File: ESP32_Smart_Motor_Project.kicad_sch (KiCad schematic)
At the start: 14 parts

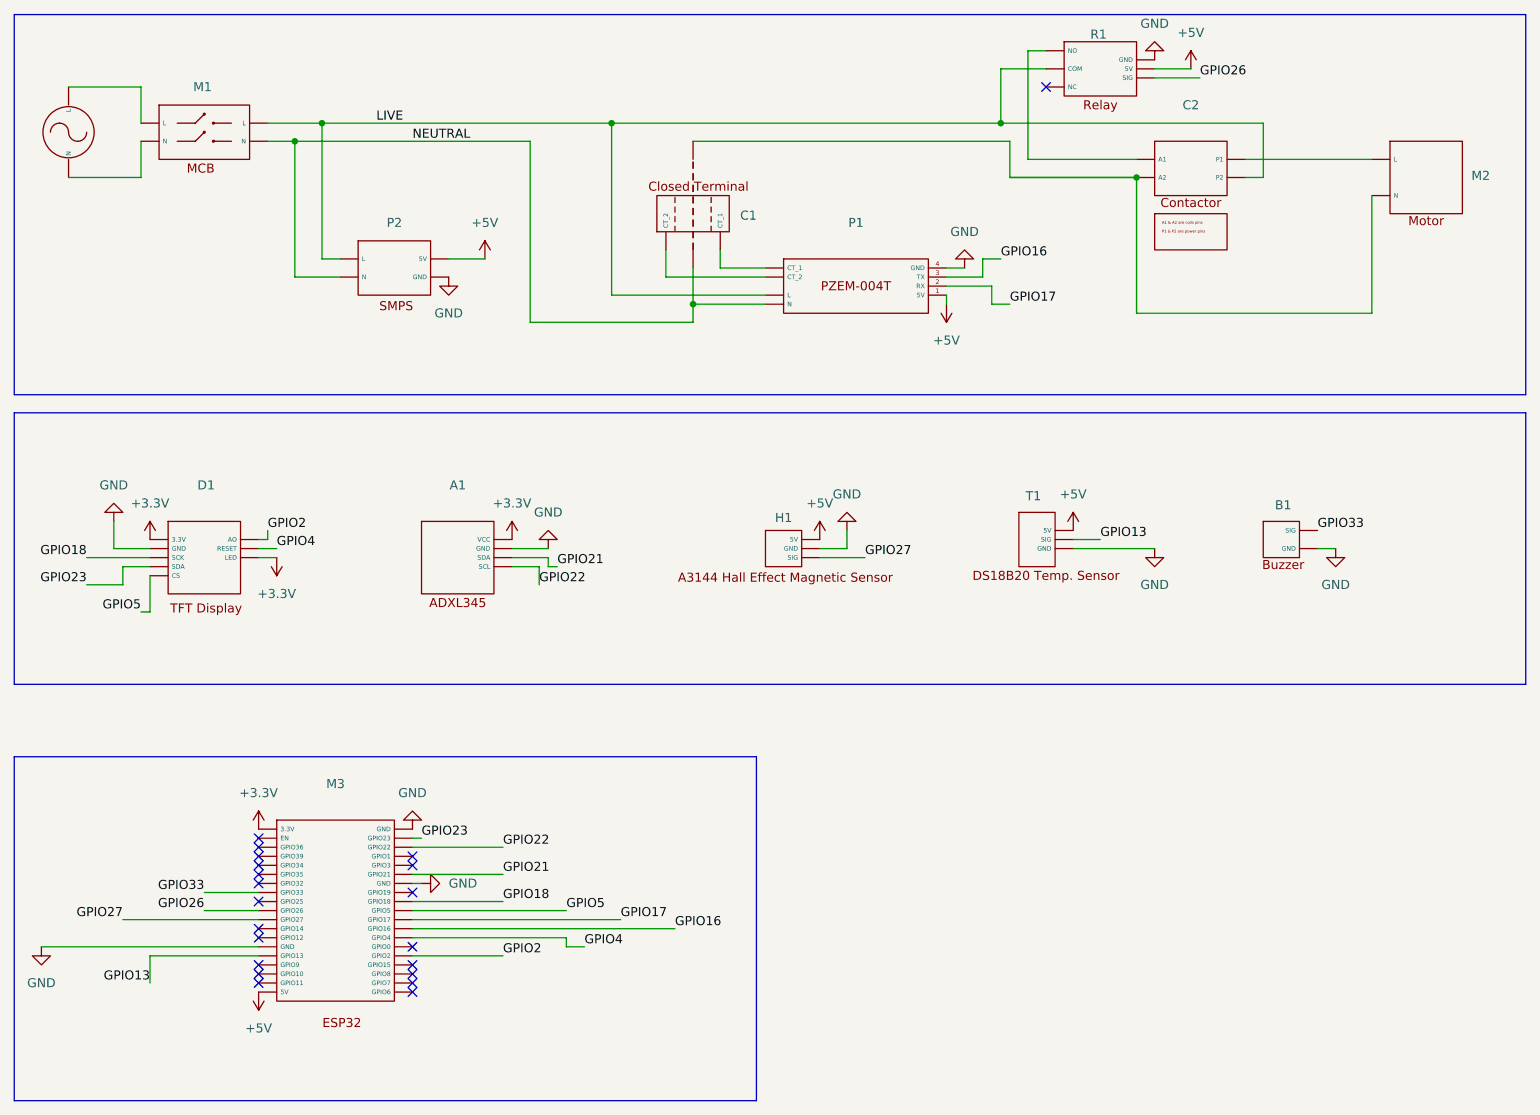
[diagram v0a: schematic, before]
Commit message: pcb design for smart motor project
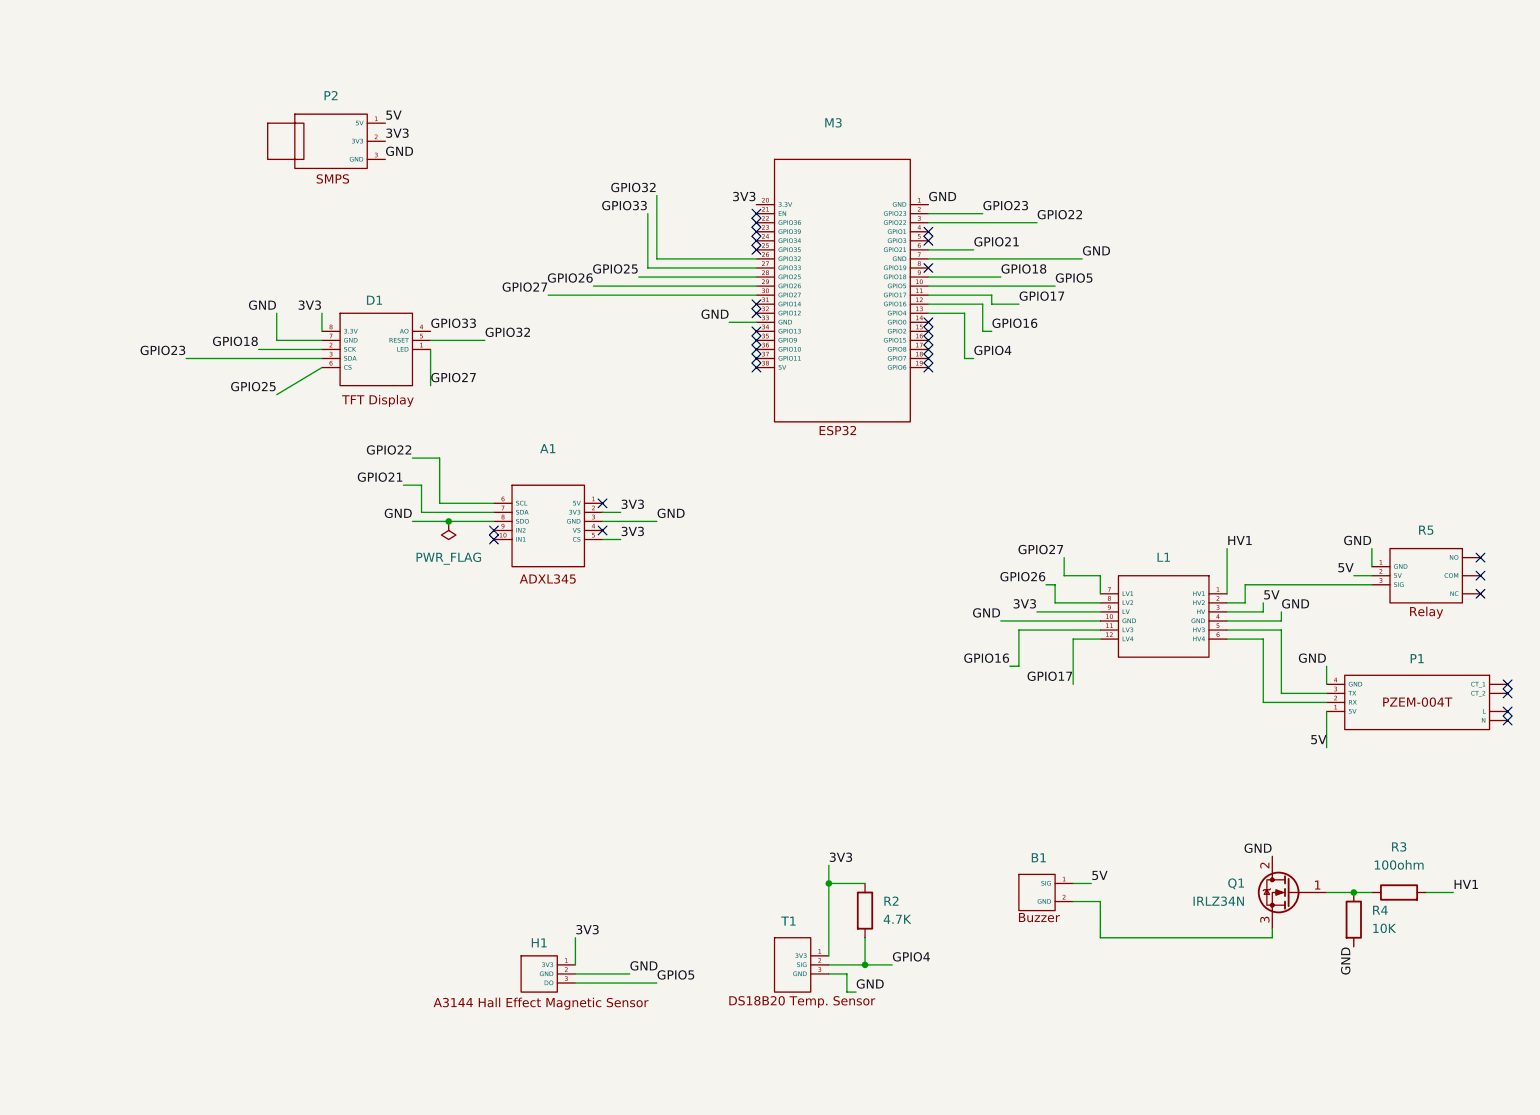
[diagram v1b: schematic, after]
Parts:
- removed C1: ~, symbol Symbol_Lib:CT
- removed C2: ~, symbol Symbol_Lib:Contactor
- removed M1: ~, symbol Symbol_Lib:MCB
- removed M2: ~, symbol Symbol_Lib:Motor
- removed R1: ~, symbol Symbol_Lib:Relay
- removed U1: ~, symbol Symbol_Lib:AC
- added L1: (no value), ESP32_Library:Logic_convertor, symbol Symbol_Lib:Level_Shifter
- added Q1: IRLZ34N, Package_TO_SOT_THT:TO-220-3_Vertical, symbol Transistor_FET:IRLZ34N
- added R2: 4.7K, Resistor_THT:R_Axial_DIN0207_L6.3mm_D2.5mm_P7.62mm_Horizontal, symbol Device:R
- added R3: 100ohm, Resistor_THT:R_Axial_DIN0207_L6.3mm_D2.5mm_P7.62mm_Horizontal, symbol Device:R
- added R4: 10K, Resistor_THT:R_Axial_DIN0207_L6.3mm_D2.5mm_P7.62mm_Horizontal, symbol Device:R
- added R5: (no value), ESP32_Library:Relay, symbol Symbol_Lib:Relay
- A1: value ~ -> (none); footprint (none) -> ESP32_Library:ADXL345
- B1: value ~ -> (none); footprint (none) -> Buzzer_Beeper:Buzzer_12x9.5RM7.6
- D1: value ~ -> (none); footprint (none) -> ESP32_Library:TFT_display
- H1: value ~ -> (none); footprint (none) -> ESP32_Library:Hall_sensor
- M3: value ~ -> (none); footprint (none) -> ESP32_Library:ESP32
- P1: value ~ -> (none); footprint (none) -> ESP32_Library:PZEM_004T
- P2: value ~ -> (none); footprint (none) -> ESP32_Library:Power_supply
- T1: value ~ -> (none); footprint (none) -> ESP32_Library:DS18B20
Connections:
- net GND: now also A1.3 (GND), A1.8 (SDO), D1.7 (GND), H1.2 (GND), M3.1 (GND), M3.33 (GND), M3.7 (GND), P2.3 (GND), T1.3 (GND), L1.10 (GND), L1.4 (GND), Q1.2 (D), R4.2, R5.1 (GND); no longer A1. (SCL), B1. (GND), D1. (LED), H1. (SIG), M3. (GPIO6), P2. (GND), T1. (GND)
- net GPIO16: now also M3.12 (GPIO16), L1.11 (LV3); no longer M3. (GPIO6), P1.3 (TX)
- net GPIO17: now also M3.11 (GPIO17), L1.12 (LV4); no longer M3. (GPIO6), P1.2 (RX)
- net GPIO18: now also D1.2 (SCK), M3.9 (GPIO18); no longer D1. (LED), M3. (GPIO6)
- net GPIO21: now also A1.7 (SDA), M3.6 (GPIO21); no longer A1. (SCL), M3. (GPIO6)
- net GPIO22: now also A1.6 (SCL), M3.3 (GPIO22); no longer A1. (SCL), M3. (GPIO6)
- net GPIO23: now also D1.3 (SDA), M3.2 (GPIO23); no longer D1. (LED), M3. (GPIO6)
- net GPIO26: now also M3.29 (GPIO26), L1.8 (LV2); no longer M3. (GPIO6)
- net GPIO27: now also D1.1 (LED), M3.30 (GPIO27), L1.7 (LV1); no longer H1. (SIG), M3. (GPIO6)
- net GPIO33: now also D1.4 (AO), M3.27 (GPIO33); no longer B1. (GND), M3. (GPIO6)
- net GPIO4: now also M3.13 (GPIO4), T1.2 (SIG), R2.2; no longer D1. (LED), M3. (GPIO6)
- net GPIO5: now also H1.3 (DO), M3.10 (GPIO5); no longer D1. (LED), M3. (GPIO6)
- removed net +3.3V: A1. (SCL), D1. (LED), M3. (GPIO6)
- removed net +5V: H1. (SIG), M3. (GPIO6), P1.1 (5V), P2. (GND), T1. (GND)
- removed net GPIO13: M3. (GPIO6), T1. (GND)
- removed net GPIO2: D1. (LED), M3. (GPIO6)
- removed net LIVE: P1. (N), P2. (GND)
- removed net NEUTRAL: P1. (N), P2. (GND)
- new net: L1.2 (HV2), R5.3 (SIG)
- new net: B1.2 (GND), Q1.3 (S)
- new net: Q1.1 (G), R3.1, R4.1
- new net: L1.5 (HV3), P1.3 (TX)
- new net: L1.6 (HV4), P1.2 (RX)
- new net 3V3: A1.2 (3V3), A1.5 (CS), D1.8 (3.3V), H1.1 (3V3), L1.9 (LV), M3.20 (3.3V), P2.2 (3V3), R2.1, T1.1 (3V3)
- new net 5V: B1.1 (SIG), L1.3 (HV), P1.1 (5V), P2.1 (5V), R5.2 (5V)
- new net GPIO25: D1.6 (CS), M3.28 (GPIO25)
- new net GPIO32: D1.5 (RESET), M3.26 (GPIO32)
- new net HV1: L1.1 (HV1), R3.2
- now unconnected: P1. (N)
- no-connect marks 21 -> 32
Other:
- moved on the sheet: P1
